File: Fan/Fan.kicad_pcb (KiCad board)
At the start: 2 copper layers, 32.5 x 14.5 mm, 25 parts, among them Q1 Hum Sensor, U2 HEF4093B

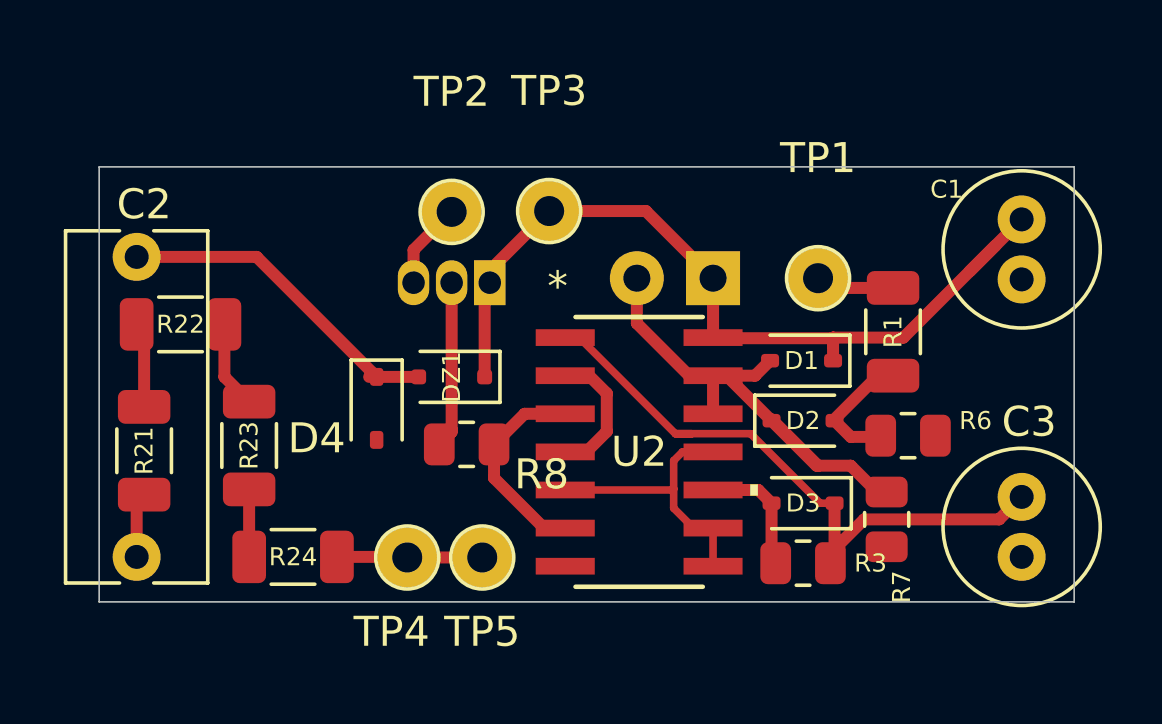
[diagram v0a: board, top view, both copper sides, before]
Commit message: pcb finnished, awaitng feedback
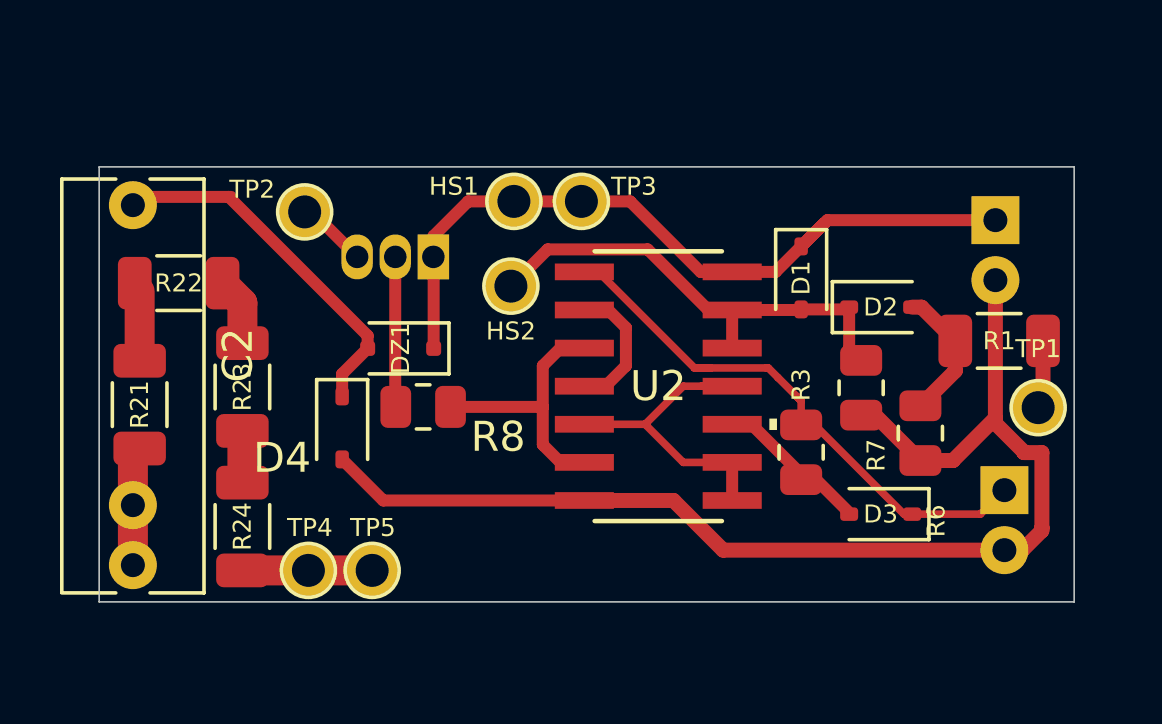
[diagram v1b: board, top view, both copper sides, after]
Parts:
- removed Q1: Hum Sensor, LED_THT:LED_D5.0mm_Clear
- added HS1: TestPoint, Pads:TestPoint_Top_Hole_D1.8x1.1mm, F.Cu at (114.3, 53.1)
- added HS2: TestPoint, Pads:TestPoint_Top_Hole_D1.8x1.1mm, F.Cu at (114.2, 56.0)
- C1, C3: footprint Capacitor_THT:C_Radial_D5.0mm_H11.0mm_P2.00mm -> Capacitors:C_Radial_D5.0mm_H11.0mm_P2.00mm_Lying; moved to B.Cu
- C2: footprint Capacitor_THT:C_Rect_L11.5mm_W4.5mm_P10.00mm_MKT -> Capacitors:C_Rect_L11.5mm_W4.5mm_P10.00mm_MKT_DoublePad
- TP1, TP2, TP3, TP4, TP5: footprint Pads:TestPoint_Top_Hole_D2.0mm -> Pads:TestPoint_Top_Hole_D1.8x1.1mm
- moved TP1 8.51 mm to (131.8, 60.0)
- moved TP2 4.90 mm to (107.3, 53.5)
- moved D2 4.58 mm to (126.5, 56.7)
- moved R7 4.47 mm to (125.9, 59.4)
- moved R3 3.70 mm to (123.9, 61.5), turned to 90 degrees
- moved TP5 3.70 mm to (109.6, 65.5)
- moved R1 3.55 mm to (130.5, 57.8), turned to 180 degrees
- moved TP4 3.32 mm to (107.5, 65.5)
- moved D1 2.76 mm to (123.9, 55.7), turned to -90 degrees
- moved D3 2.61 mm to (126.5, 63.6)
- moved U2 2.28 mm to (119.1, 59.3)
- moved D5 2.07 mm to (111.6, 55.0)
- moved R24 1.97 mm to (105.3, 64.0), turned to 90 degrees
- moved R23 1.96 mm to (105.3, 59.3)
- moved DZ1 1.95 mm to (110.5, 58.0)
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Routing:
- net GND: track 0.00 -> 39.9 mm
- net Net-(D3-K): track 23.1 -> 20.4 mm
- net Net-(R8-Pad1): track 6.98 -> 8.97 mm
- net +12V: track 28.7 -> 26.7 mm
- net Net-(C2-Pad2): track 2.18 -> 3.96 mm
- net Net-(D1-A): track 17.6 -> 15.9 mm
- net Net-(U2-Pad11): track 9.51 -> 11.2 mm
- net Net-(D5-G): track 6.27 -> 5.01 mm
- net Net-(D3-A): track 4.19 -> 5.23 mm
- net Net-(D5-A2): track 2.89 -> 2.12 mm
- net Net-(R22-Pad1): track 2.92 -> 2.27 mm
- net Net-(D4-K): track 11.3 -> 11.9 mm
- net Net-(R21-Pad1): track 2.85 -> 2.31 mm
- net Net-(R24-Pad1): track 4.85 -> 4.32 mm
- net Net-(R23-Pad1): track 2.25 -> 1.73 mm
